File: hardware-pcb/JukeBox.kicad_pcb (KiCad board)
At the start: 2 copper layers, 90 x 90 mm, 79 parts, among them J1 USB4105-GF-A, J2 AudioJack4_Ground, Q1 Q_NPN_ECB, SW1 SW_SPST, SW10 SW_SPST, SW11 SW_SPST, SW12 SW_SPST, SW2 SW_SPST, SW3 SW_SPST, SW4 SW_SPST, SW5 SW_SPST, SW6 SW_SPST, SW7 SW_SPST, SW8 SW_SPST, SW9 SW_SPST, U1 NCP1117-3.3_SOT223, U2 W25Q128JVS, U3 RP2040, U4 st7789v, Y1 ECS-120-20-33-AEL-TR

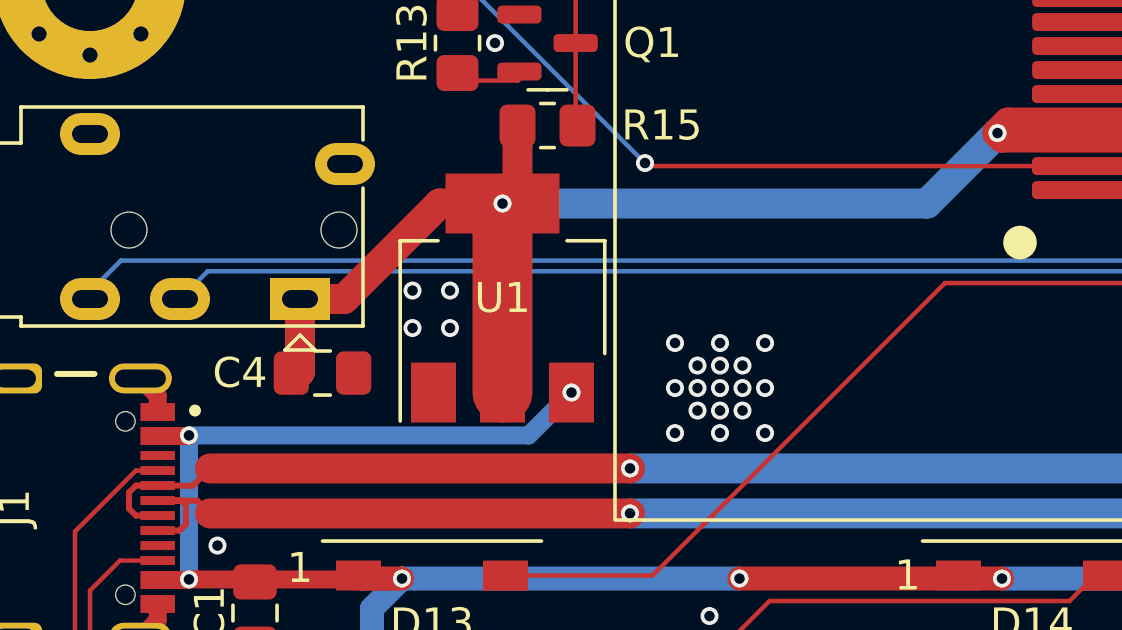
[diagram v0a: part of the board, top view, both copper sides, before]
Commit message: minor updates for production
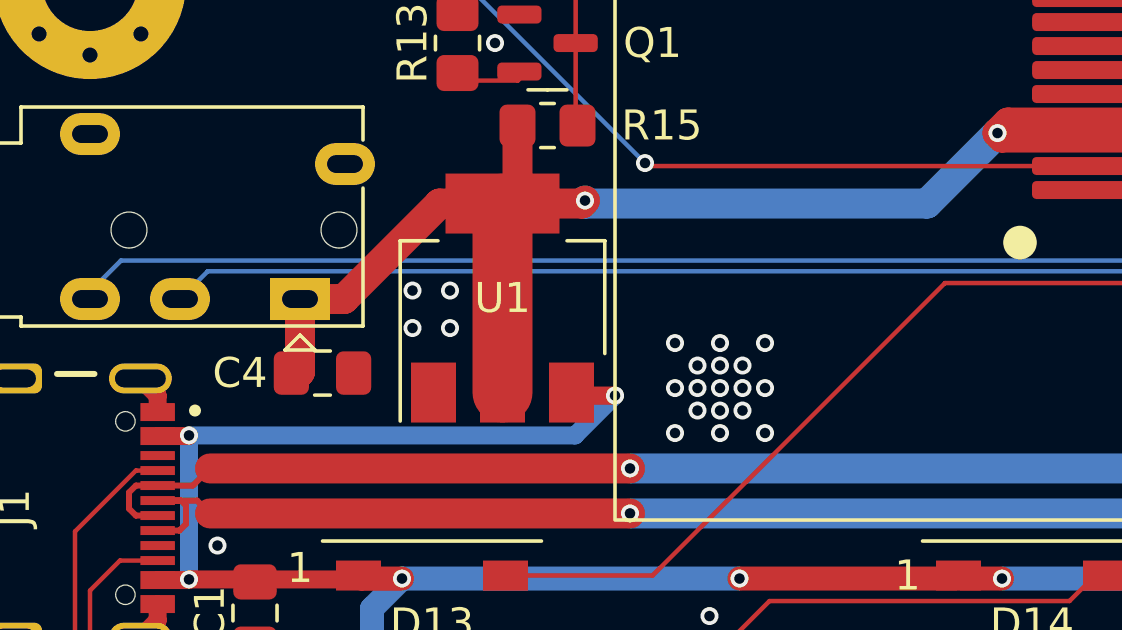
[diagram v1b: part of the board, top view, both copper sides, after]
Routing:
- net VBUS: track 250.7 -> 253.6 mm
